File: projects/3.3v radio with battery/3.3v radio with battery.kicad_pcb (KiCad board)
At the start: 2 copper layers, 130 x 90 mm, 21 parts, among them J1 USB_B

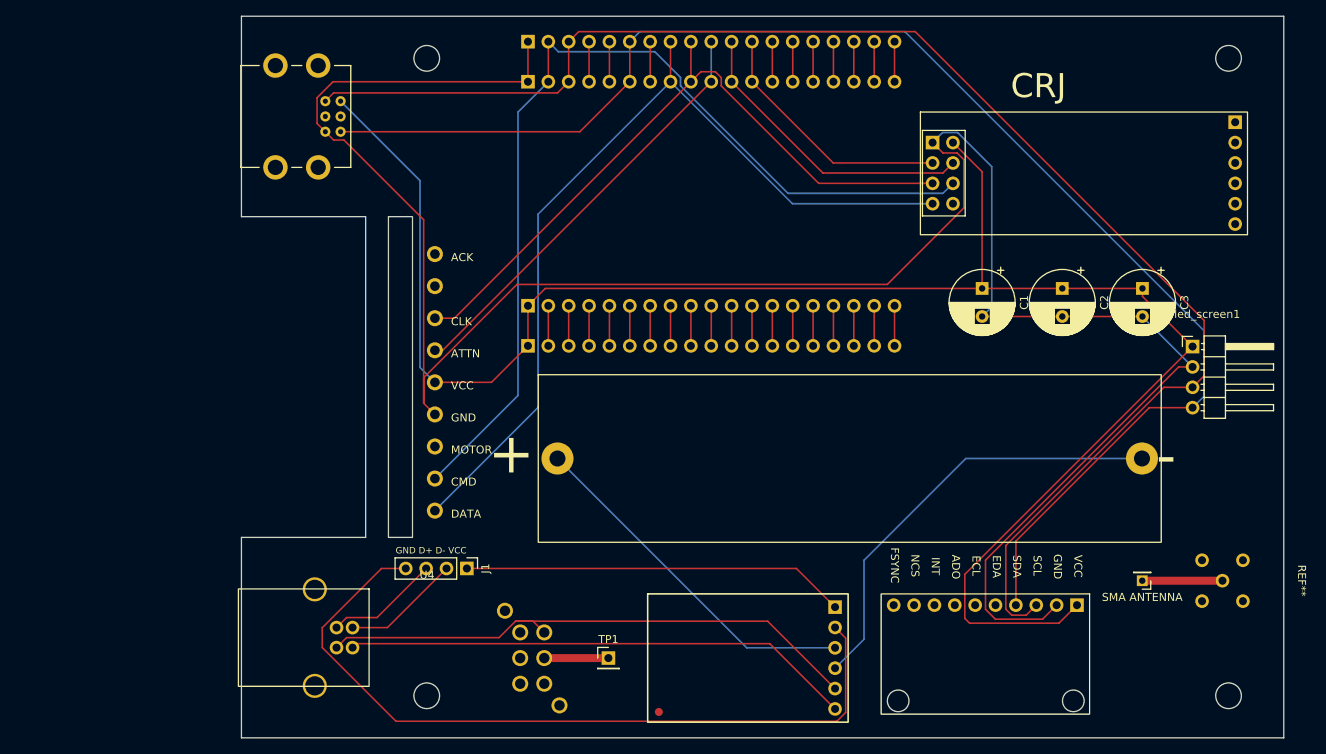
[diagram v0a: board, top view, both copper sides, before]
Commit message: only multi remote left
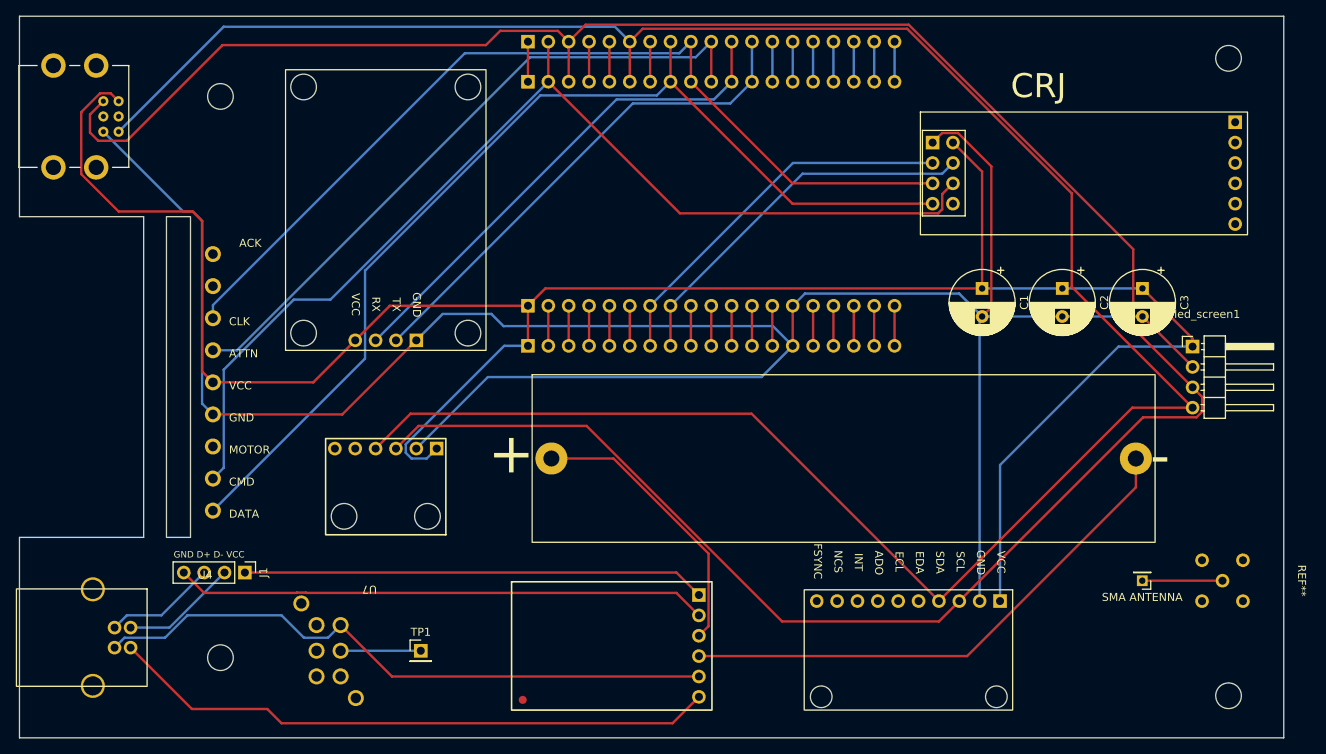
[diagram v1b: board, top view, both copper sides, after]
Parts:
- added GPS1: ~, Footprints_cez:GY-NEO6MV2_flipped, F.Cu at (102.2, 72.3)
- added U7: ~, Footprints_cez:BME280, F.Cu at (115.1, 119.7)
- moved J1 27.7 mm to (99.6, 118.1)
- moved U1 27.7 mm to (78.2, 61.2)
- moved U2 27.7 mm to (100.0, 91.1)
- moved U4 27.7 mm to (96.6, 126.1)
- moved REF** 26.2 mm to (96.5, 58.7)
- moved REF** 26.2 mm to (96.5, 128.7)
- moved U6 25.4 mm to (109.9, 115.2)
- moved TP1 23.4 mm to (121.5, 127.9)
- moved U3 17.0 mm to (144.8, 112.8)
- moved MPU1 9.61 mm to (199.9, 126.9)
- moved U5 0.76 mm to (144.1, 96.1)
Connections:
- C1 pad 2: Net-(MPU1-GND) -> Net-(GPS1-GND)
- C2 pad 2: Net-(MPU1-GND) -> Net-(GPS1-GND)
- C3 pad 2: Net-(MPU1-GND) -> Net-(GPS1-GND)
- ESP32-WROOM-32U1 pad 14: unconnected-(ESP32-WROOM-32U1-GND-Pad14) -> Net-(GPS1-GND)
- ESP32-WROOM-32U1 pad 20: Net-(MPU1-GND) -> unconnected-(ESP32-WROOM-32U1-GND-Pad20)
- ESP32-WROOM-32U1 pad 30: Net-(ESP32-WROOM-32U1-17) -> Net-(ESP32-WROOM-32U1-TX2/17)
- ESP32-WROOM-32U1 pad 31: Net-(ESP32-WROOM-32U1-16) -> Net-(ESP32-WROOM-32U1-RX2/16)
- ESP32-WROOM-32U1 pad 7: unconnected-(ESP32-WROOM-32U1-32-Pad7) -> Net-(ESP32-WROOM-32U1-32)
- ESP32-WROOM-32U1 pad 8: unconnected-(ESP32-WROOM-32U1-33-Pad8) -> Net-(ESP32-WROOM-32U1-33)
- MPU1 pad 2: Net-(MPU1-GND) -> Net-(GPS1-GND)
- NRF1 pad 1: Net-(MPU1-GND) -> Net-(GPS1-GND)
- NRF1 pad 3: Net-(ESP32-WROOM-32U1-16) -> Net-(ESP32-WROOM-32U1-32)
- NRF1 pad 4: Net-(ESP32-WROOM-32U1-17) -> Net-(ESP32-WROOM-32U1-33)
- Oled_screen1 pad 2: Net-(MPU1-GND) -> Net-(GPS1-GND)
- U1 pad 6: Net-(MPU1-GND) -> Net-(GPS1-GND)
- U2 pad 4: Net-(MPU1-GND) -> Net-(GPS1-GND)
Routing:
- net Net-(GPS1-GND): track 0.00 -> 296.7 mm
- net Net-(MPU1-GND): track 278.3 -> 0.00 mm
- net Net-(ESP32-WROOM-32U1-SCL/22): track 184.0 -> 305.3 mm
- net Net-(ESP32-WROOM-32U1-SDA/21): track 178.3 -> 295.6 mm
- net Net-(ESP32-WROOM-32U1-TX2/17): track 0.00 -> 62.8 mm
- net Net-(ESP32-WROOM-32U1-RX2/16): track 0.00 -> 62.8 mm
- net Net-(ESP32-WROOM-32U1-3.3v): track 226.3 -> 280.4 mm
- net Net-(ESP32-WROOM-32U1-33): track 0.00 -> 47.6 mm
- net Net-(ESP32-WROOM-32U1-32): track 0.00 -> 47.6 mm
- net Net-(ESP32-WROOM-32U1-17): track 37.8 -> 0.00 mm
- net Net-(ESP32-WROOM-32U1-16): track 31.7 -> 0.00 mm
- net Net-(J1-GND): track 96.6 -> 66.5 mm
- net Net-(ESP32-WROOM-32U1-SS/5): track 53.3 -> 83.1 mm
- net Net-(ESP32-WROOM-32U1-SCK/18): track 86.2 -> 115.2 mm
- net Net-(ESP32-WROOM-32U1-MISO/19): track 109.7 -> 129.6 mm
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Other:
- board size 130 x 90 mm -> 157.7 x 90 mm
- board text added: "+"
